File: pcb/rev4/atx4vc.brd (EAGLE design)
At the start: 69 x 69 mm, 48 parts, among them IC1 MY_7905DT, J2 ATX24RH

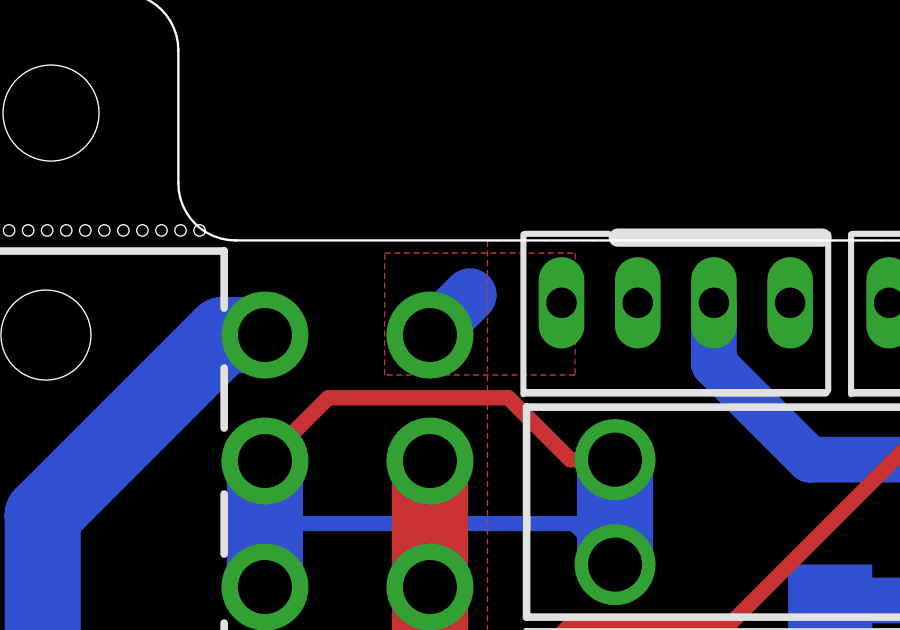
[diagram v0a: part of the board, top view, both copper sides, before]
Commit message: working on update
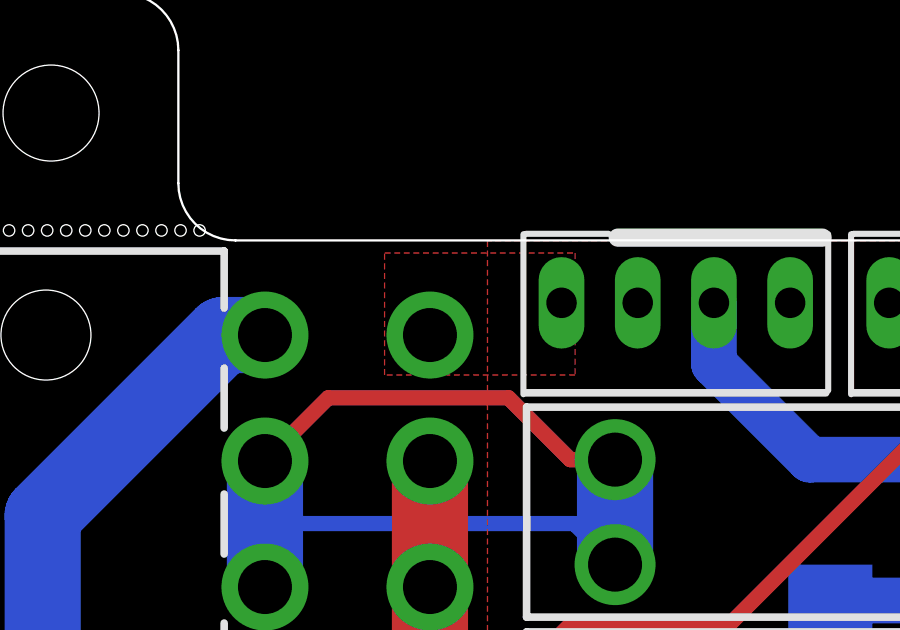
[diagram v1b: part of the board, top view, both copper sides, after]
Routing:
- net GND: track 100.5 -> 98.6 mm
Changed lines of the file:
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@@
 <contactref element="U$12" pad="P$4"/>
 <contactref element="JP4" pad="1"/>
-<polygon width="0.1524" layer="1">
+<polygon width="0.1524" layer="1" isolate="0.4064">
 <vertex x="15.0895" y="38.235"/>
 <vertex x="15.0895" y="26.297"/>
@@
 <wire x1="10.1565" y1="19.8" x2="11.1965" y2="19.8" width="1.778" layer="1"/>
 <wire x1="11.1965" y1="19.8" x2="16.6965" y2="19.8" width="1.778" layer="1"/>
-<wire x1="16.6965" y1="57.6" x2="18.0325" y2="58.936" width="1.778" layer="16"/>
 <wire x1="7.5965" y1="34.298" x2="7.5965" y2="28.202" width="1.778" layer="1"/>
 <wire x1="7.5965" y1="28.202" x2="7.5965" y2="22.36" width="1.778" layer="1"/>
@@
 <vertex x="67.6355" y="10.041"/>
 </polygon>
-<polygon width="0.1524" layer="1" thermals="no">
+<polygon width="0.1524" layer="1" isolate="0.4064" thermals="no">
 <vertex x="21.5345" y="56.269"/>
 <vertex x="15.1845" y="56.269"/>
@@
 <vertex x="57.4755" y="14.105"/>
 </polygon>
-<polygon width="0.1524" layer="1" thermals="no">
+<polygon width="0.1524" layer="1" isolate="0.4064" thermals="no">
 <vertex x="23.3125" y="18.423"/>
 <vertex x="14.9305" y="18.423"/>
